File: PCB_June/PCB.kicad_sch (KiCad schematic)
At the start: 26 parts, among them J2 FH34SRJ-24S-0.5SH_99_, J9 61302421121, Q1 BSS138, Q2 S8050, U3 AO3401

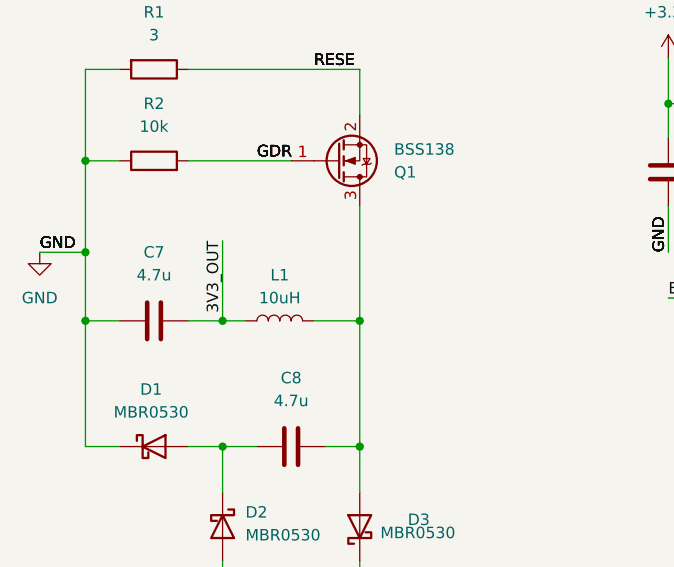
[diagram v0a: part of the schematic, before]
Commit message: claire can i get inductor footprint haha
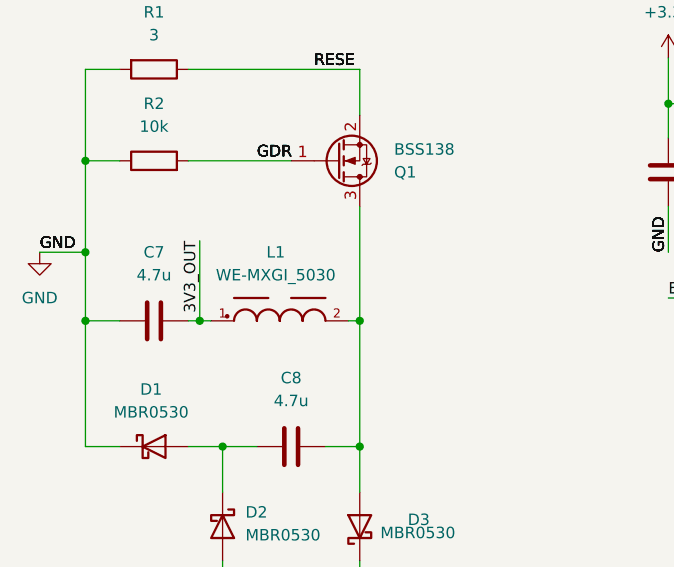
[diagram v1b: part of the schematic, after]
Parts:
- removed L1: 10uH, Inductor_SMD:L_0805_2012Metric_Pad1.05x1.20mm_HandSolder, symbol Device:L
- added L1: WE-MXGI_5030, WE-MXGI_5030:WE-MXGI_5030, symbol WE-MXGI_5030:WE-MXGI_5030
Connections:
- net 3V3_OUT: now also L1.1
- net at C8.2, D3.2 (A), Q1.3 (D): now also L1.2
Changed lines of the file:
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@@
 	)
 	(junction
-		(at 110.49 48.26)
+		(at 34.29 50.8)
 		(diameter 0)
 		(color 0 0 0 0)
 	)
 	(junction
-		(at 121.92 60.96)
+		(at 110.49 48.26)
 		(diameter 0)
 		(color 0 0 0 0)
 	)
 	(junction
-		(at 22.86 161.29)
+		(at 52.07 50.8)
 		(diameter 0)
 		(color 0 0 0 0)
 	)
 	(junction
-		(at 96.52 153.67)
+		(at 121.92 60.96)
 		(diameter 0)
 		(color 0 0 0 0)
 	)
 	(junction
-		(at 52.07 50.8)
+		(at 22.86 161.29)
 		(diameter 0)
 		(color 0 0 0 0)
 	)
 	(junction
-		(at 121.92 40.64)
+		(at 96.52 153.67)
 		(diameter 0)
 		(color 0 0 0 0)
 	)
 	(junction
-		(at 36.83 50.8)
+		(at 121.92 40.64)
 		(diameter 0)
 		(color 0 0 0 0)
@@
 	(wire
 		(pts
-			(xy 21.59 50.8) (xy 21.59 64.77)
+			(xy 52.07 50.8) (xy 52.07 64.77)
 		)
 		(stroke
@@
 	(wire
 		(pts
-			(xy 53.34 151.13) (xy 71.12 151.13)
+			(xy 21.59 50.8) (xy 21.59 64.77)
 		)
 		(stroke
@@
 	(wire
 		(pts
-			(xy 53.34 130.81) (xy 73.66 130.81)
+			(xy 53.34 151.13) (xy 71.12 151.13)
 		)
 		(stroke
@@
 	(wire
 		(pts
-			(xy 78.74 158.75) (xy 96.52 158.75)
+			(xy 53.34 130.81) (xy 73.66 130.81)
 		)
 		(stroke
@@
 	(wire
 		(pts
-			(xy 36.83 77.47) (xy 36.83 83.82)
+			(xy 78.74 158.75) (xy 96.52 158.75)
 		)
 		(stroke
@@
 	(wire
 		(pts
-			(xy 107.95 26.67) (xy 107.95 29.21)
+			(xy 36.83 77.47) (xy 36.83 83.82)
 		)
 		(stroke
@@
 	(wire
 		(pts
-			(xy 46.99 50.8) (xy 52.07 50.8)
+			(xy 107.95 26.67) (xy 107.95 29.21)
 		)
 		(stroke
@@
 	(wire
 		(pts
-			(xy 36.83 50.8) (xy 39.37 50.8)
-		)
-		(stroke
-			(width 0)
-			(type default)
-		)
-	)
-	(wire
-		(pts
 			(xy 21.59 43.18) (xy 21.59 50.8)
 		)
@@
 	(wire
 		(pts
-			(xy 33.02 50.8) (xy 36.83 50.8)
+			(xy 33.02 50.8) (xy 34.29 50.8)
 		)
 		(stroke
@@
 	(wire
 		(pts
+			(xy 34.29 50.8) (xy 35.56 50.8)
+		)
+		(stroke
+			(width 0)
+			(type default)
+		)
+	)
+	(wire
+		(pts
 			(xy 111.76 119.38) (xy 119.38 119.38)
 		)
@@
 	(wire
 		(pts
-			(xy 52.07 50.8) (xy 52.07 64.77)
+			(xy 124.46 26.67) (xy 130.81 26.67)
 		)
 		(stroke
@@
 	(wire
 		(pts
-			(xy 124.46 26.67) (xy 130.81 26.67)
+			(xy 33.02 64.77) (xy 36.83 64.77)
 		)
 		(stroke
@@
 	(wire
 		(pts
-			(xy 33.02 64.77) (xy 36.83 64.77)
+			(xy 34.29 41.91) (xy 34.29 50.8)
 		)
 		(stroke
@@
 	(wire
 		(pts
-			(xy 36.83 41.91) (xy 36.83 50.8)
+			(xy 121.92 31.75) (xy 121.92 40.64)
 		)
 		(stroke
@@
 	(wire
 		(pts
-			(xy 121.92 31.75) (xy 121.92 40.64)
+			(xy 52.07 77.47) (xy 52.07 83.82)
 		)
 		(stroke
@@
 	(wire
 		(pts
-			(xy 52.07 77.47) (xy 52.07 83.82)
+			(xy 50.8 50.8) (xy 52.07 50.8)
 		)
 		(stroke
@@
 	)
 	(label "3V3_OUT"
-		(at 36.83 41.91 270)
+		(at 34.29 41.91 270)
 		(effects
 			(font
@@
 	)
 	(symbol
+		(lib_id "WE-MXGI_5030:WE-MXGI_5030")
+		(at 43.18 50.8 0)
+		(unit 1)
+		(exclude_from_sim no)
+		(in_bom yes)
+		(on_board yes)
+		(dnp no)
+		(fields_autoplaced yes)
+		(property "Reference" "L1"
+			(at 42.7355 43.18 0)
+			(effects
+				(font
+					(size 1.27 1.27)
+				)
+			)
+		)
+		(property "Value" "WE-MXGI_5030"
+			(at 42.7355 45.72 0)
+			(effects
+				(font
+					(size 1.27 1.27)
+				)
+			)
+		)
+		(property "Footprint" "WE-MXGI_5030:WE-MXGI_5030"
+			(at 43.18 50.8 0)
+			(effects
+				(font
+					(size 1.27 1.27)
+				)
+				(justify bottom)
+				(hide yes)
+			)
+		)
+		(property "Datasheet" ""
+			(at 43.18 50.8 0)
+			(effects
+				(font
+					(size 1.27 1.27)
+				)
+				(hide yes)
+			)
+		)
+		(property "Description" ""
+			(at 43.18 50.8 0)
+			(effects
+				(font
+					(size 1.27 1.27)
+				)
+				(hide yes)
+			)
+		)
+		(pin "1"
+		)
+		(pin "2"
+		)
+		(instances
+			(project ""
+				(path "/8dcae476-bf02-4dea-8567-670805b7ab7c/9f33d424-8f8c-499b-911f-2b5f72ba0270"
+					(reference "L1")
+					(unit 1)
+				)
+			)
+		)
+	)
+	(symbol
 		(lib_id "Device:C")
 		(at 74.93 161.29 90)
@@
 					(unit 1)
 				)
-			)
-		)
-	)
-	(symbol
-		(lib_id "Device:L")
-		(at 43.18 50.8 90)
-		(unit 1)
-		(exclude_from_sim no)
-		(in_bom yes)
-		(on_board yes)
-		(dnp no)
-		(fields_autoplaced yes)
-		(property "Reference" "L1"
-			(at 43.18 45.72 90)
-			(effects
-				(font
-					(size 1.27 1.27)
-				)
-			)
-		)
-		(property "Value" "10uH"
-			(at 43.18 48.26 90)
-			(effects
-				(font
-					(size 1.27 1.27)
-				)
-			)
-		)
-		(property "Footprint" "Inductor_SMD:L_0805_2012Metric_Pad1.05x1.20mm_HandSolder"
-			(at 43.18 50.8 0)
-			(effects
-				(font
-					(size 1.27 1.27)
-				)
-				(hide yes)
-			)
-		)
-		(property "Datasheet" "~"
-			(at 43.18 50.8 0)
-			(effects
-				(font
-					(size 1.27 1.27)
-				)
-				(hide yes)
-			)
-		)
-		(property "Description" "Inductor"
-			(at 43.18 50.8 0)
-			(effects
-				(font
-					(size 1.27 1.27)
-				)
-				(hide yes)
-			)
-		)
-		(pin "2"
-		)
-		(pin "1"
-		)
-		(instances
-			(project ""
-				(path "/4d36fe0e-b49e-45a2-8e76-66c0323912e5"
-					(reference "L201")
-					(unit 1)
-				)
-			)
-			(project "EE 447"
-				(path "/8dcae476-bf02-4dea-8567-670805b7ab7c/9f33d424-8f8c-499b-911f-2b5f72ba0270"
-					(reference "L1")
-					(unit 1)
-				)
